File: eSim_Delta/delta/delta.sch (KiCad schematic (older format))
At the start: 42 parts, among them U1 plot_v1, U10 plot_v1, U11 plot_v1, U2 ashwini_delay1bit, U3 adc_bridge_5, U4 dac_bridge_2, U5 plot_v1, U6 plot_v1, U7 plot_v1, U9 plot_v1, X1 avsd_opamp, X2 avsd_opamp, X3 avsd_opamp, X4 avsd_opamp, X5 avsd_opamp, X6 avsd_opamp

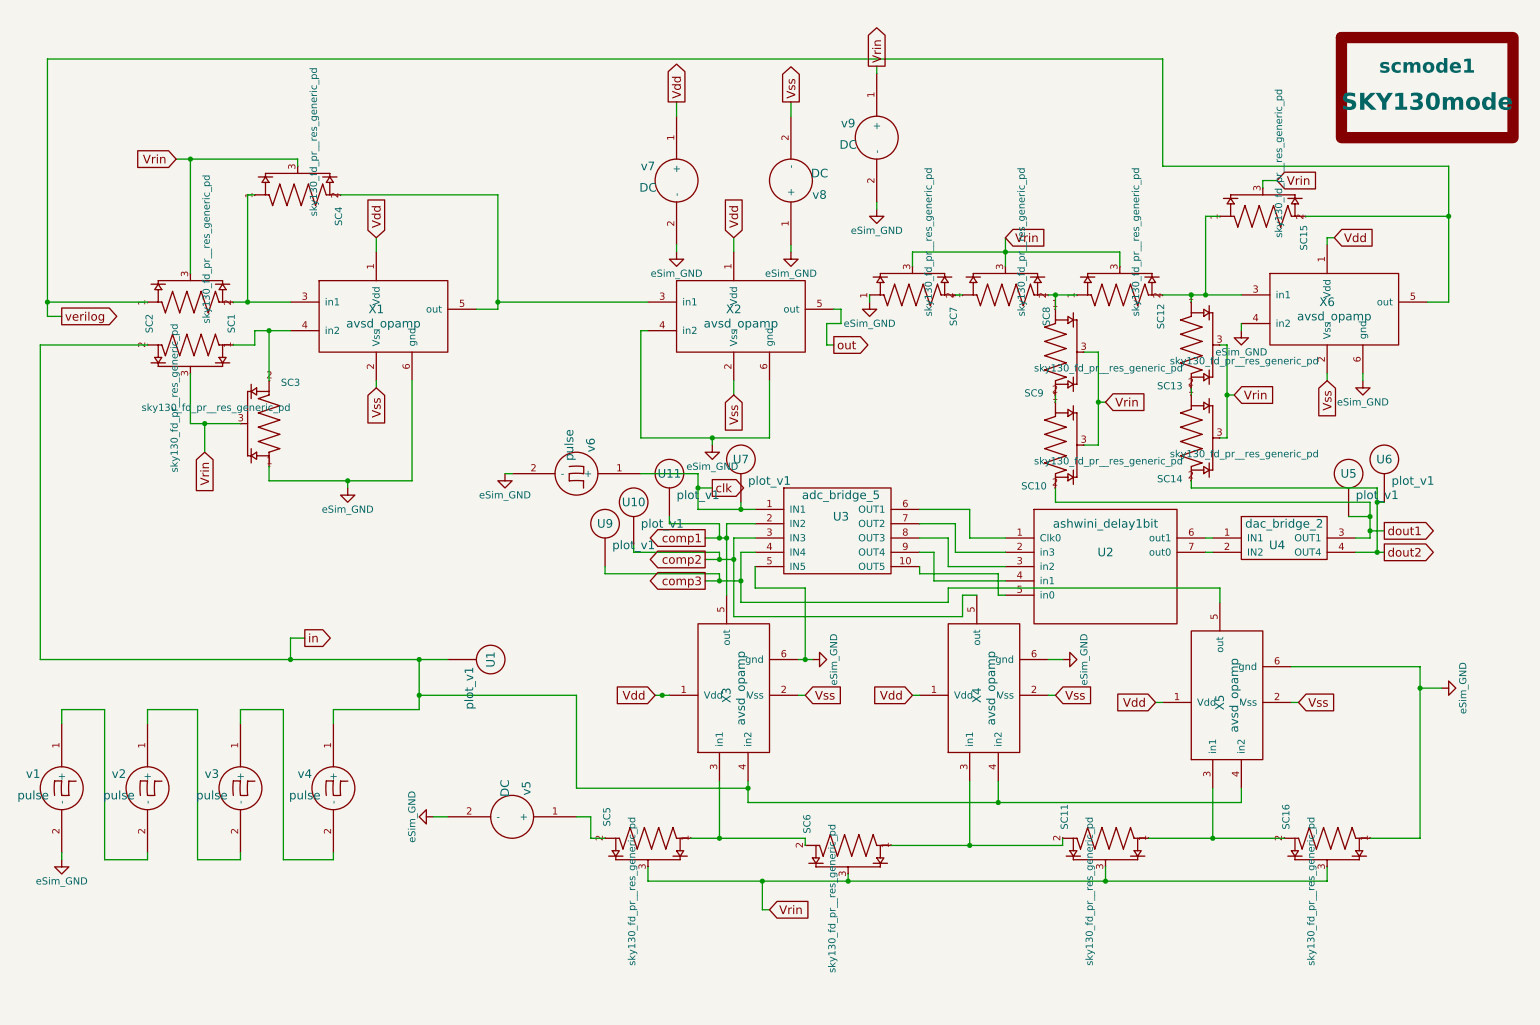
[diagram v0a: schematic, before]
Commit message: final
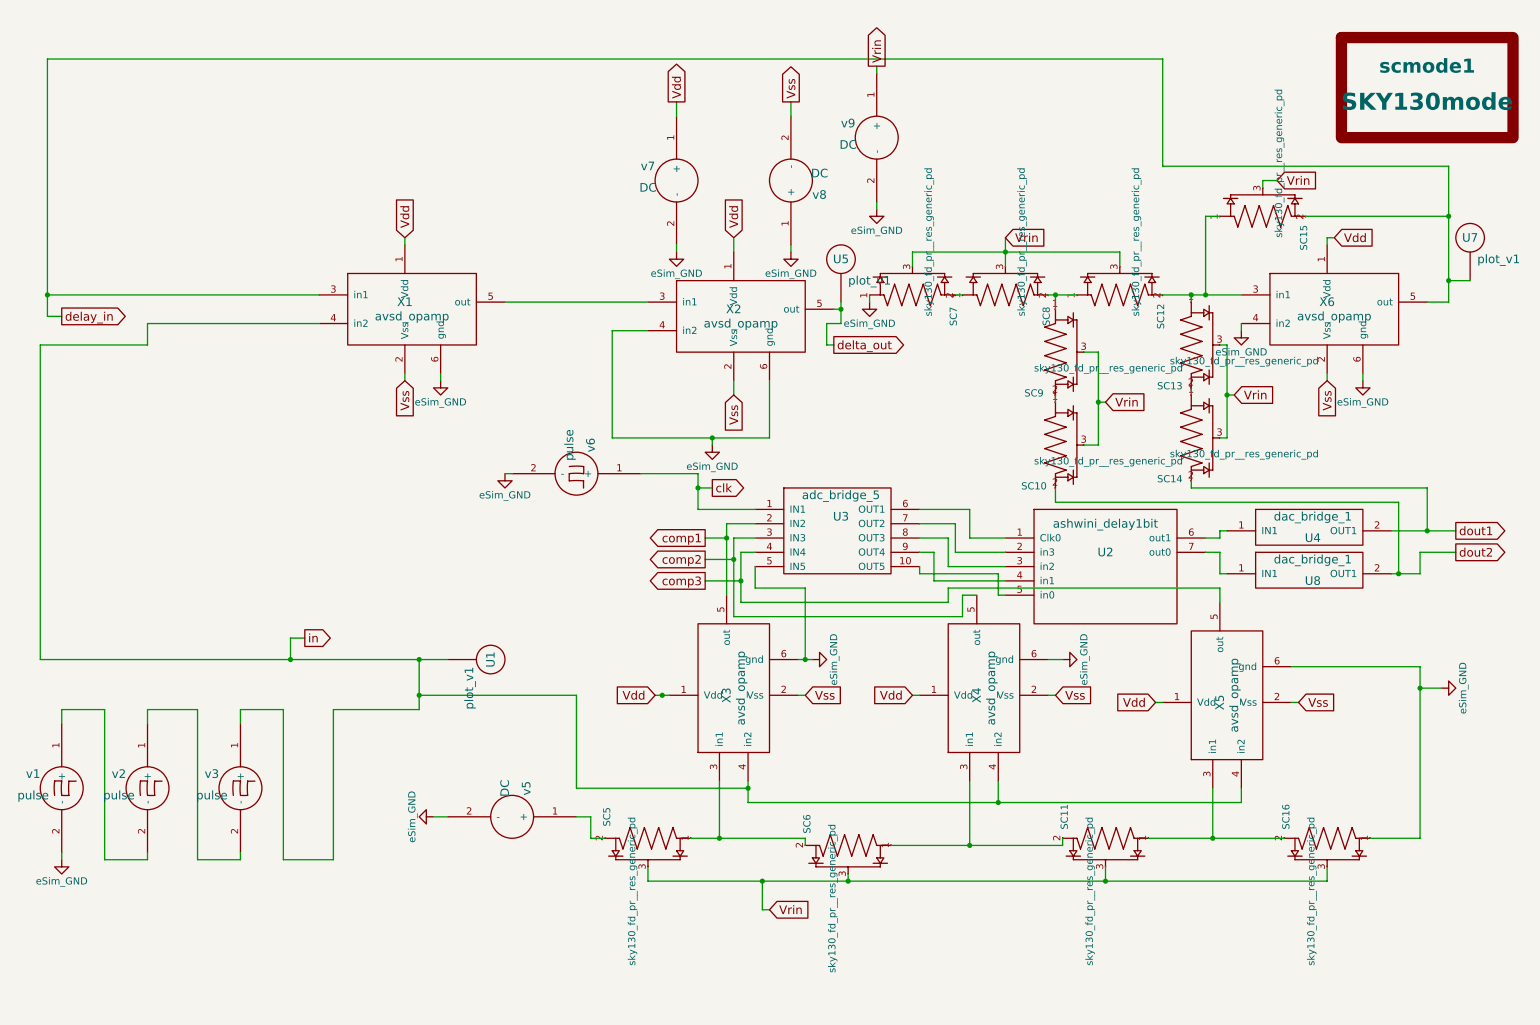
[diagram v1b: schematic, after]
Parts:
- removed SC1, SC2, SC3, SC4: sky130_fd_pr__res_generic_pd, symbol sky130_fd_pr__res_generic_pd
- removed U10, U11, U6, U9: plot_v1, symbol plot_v1
- removed U4: dac_bridge_2, symbol dac_bridge_2
- removed v4: pulse, symbol pulse
- added U4, U8: dac_bridge_1, symbol dac_bridge_1
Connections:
- net verilog is gone; now on net delay_in: SC15.2 (P), X6.5 (out)
- net clk: no longer U7.~
- net dout1: now also SC14.2 (P), U4.2 (OUT1); no longer SC10.2 (P), U5.~
- net dout2: now also SC10.2 (P), U8.2 (OUT1); no longer SC14.2 (P)
- net in: now also X1.4 (in2), v3.1 (+)
- net delay_in: now reaches X1.3 (in1)
- net delay_in: now also U7.~
- net at U2.6 (out1): now also U4.1 (IN1)
- net at U2.7 (out0): now also U8.1 (IN1)
- net out renamed delta_out
- net delta_out: now also U5.~
